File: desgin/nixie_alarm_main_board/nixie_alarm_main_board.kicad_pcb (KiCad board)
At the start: 2 copper layers, 138.2 x 53 mm, 105 parts, among them IC1 LM3488MM, IC2 HV5530PG-G, IC3 TPS563219ADDFR, IC4 HV5530PG-G, IC6 CD40109BQNSRQ1, IC7 AP7363-33D-13, IC8 MCP4018T-502E_LT, J1 PJ-094H-SMT-TR, J2 JST XH 2.54 3 pin, J3 USB_C_Receptacle_USB2.0_16P, Q1 SSM3K35AMFV,L3F, Q2 DMN60H080DS-13, Q3 DMN60H080DS-13, Q4 DMN60H080DS-13, Q5 DMN60H080DS-13, Q6 DMN60H080DS-13, Q7 DMN60H080DS-13, Q8 TPH5200FNH,L1Q, U1 ESP32-S3-WROOM-1

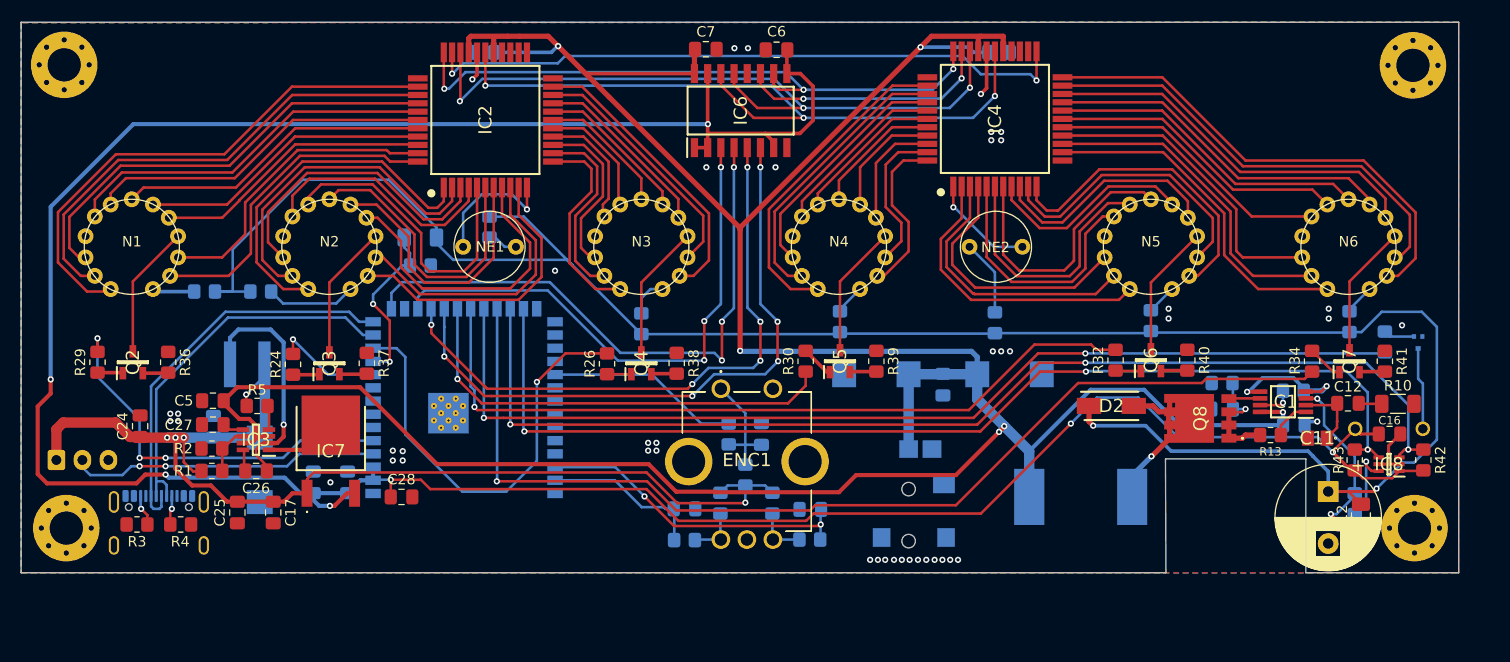
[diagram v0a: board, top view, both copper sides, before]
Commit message: add more detalis
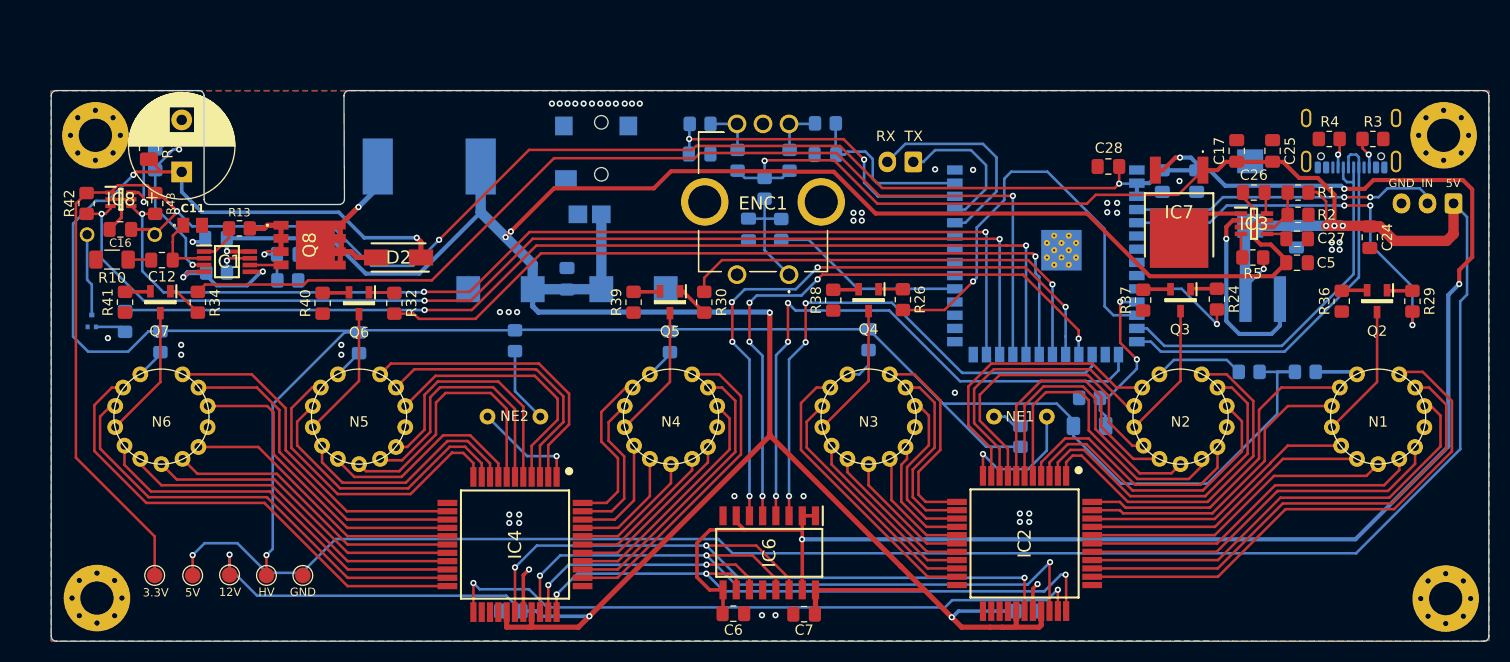
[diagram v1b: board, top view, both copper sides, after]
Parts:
- added 12V: TestPoint_Pad_D1.5mm, TestPoint:TestPoint_Pad_D1.5mm, F.Cu at (104.0, 120.2)
- added 3.3V: TestPoint_Pad_D1.5mm, TestPoint:TestPoint_Pad_D1.5mm, F.Cu at (96.8, 120.2)
- added 5V: TestPoint_Pad_D1.5mm, TestPoint:TestPoint_Pad_D1.5mm, F.Cu at (100.5, 120.2)
- added GND: TestPoint_Pad_D1.5mm, TestPoint:TestPoint_Pad_D1.5mm, F.Cu at (111.0, 120.2)
- added HV: TestPoint_Pad_D1.5mm, TestPoint:TestPoint_Pad_D1.5mm, F.Cu at (107.5, 120.2)
- added J4: JST XH 2.54 3 pin, Connector_JST:JST_EH_S2B-EH_1x02_P2.50mm_Horizontal, B.Cu at (169.8, 80.4)
- moved REF** 142.4 mm to (220.9, 122.4), turned to 180 degrees
- moved REF** 137.7 mm to (220.8, 77.9), turned to 180 degrees
- moved J2 136.6 mm to (221.7, 84.4), turned to 180 degrees
- moved REF** 136.5 mm to (91.2, 122.4), turned to 180 degrees
- moved REF** 132.4 mm to (91.1, 77.9), turned to 180 degrees
- moved R42 130.9 mm to (90.2, 84.4), turned to 90 degrees
- moved Q1 127.6 mm to (90.8, 95.7), turned to 180 degrees
- moved R29 126.6 mm to (217.8, 93.8), turned to -90 degrees
- moved IC8 124.6 mm to (93.5, 84.0), turned to 0 degrees
- moved R3 124.5 mm to (213.9, 78.2), turned to 0 degrees
- moved R10 124.4 mm to (92.7, 89.8), turned to 180 degrees
- moved C16 123.6 mm to (93.5, 86.9), turned to 180 degrees
- moved LS1 123.4 mm to (93.5, 87.4), turned to 180 degrees
- moved R12 122.1 mm to (96.2, 78.6), turned to 90 degrees
- moved R41 121.3 mm to (94.0, 93.9), turned to 90 degrees
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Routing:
- net +5V: track 111.0 -> 267.2 mm, vias 5 -> 6
- net +3.3V: track 282.8 -> 322.0 mm
- net +12V: track 288.7 -> 322.0 mm, vias 6 -> 7
- net HV: track 201.9 -> 229.7 mm, vias 2 -> 3
- net DEBUG_UART_RX: track 0.00 -> 20.3 mm
- net DEBUG_UART_TX: track 0.00 -> 14.2 mm
- net ENC_A: track 16.0 -> 17.3 mm
- net ENC_B: track 30.6 -> 31.8 mm
- net NX_DOT_6: track 101.7 -> 100.9 mm
- net GND: vias 47 -> 53
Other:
- outline, holes or cut-outs redrawn
- board text added: "5V"
- board text added: "GND"
- board text added: "HV Danger"
- board text added: "IN"
- board text added: "Nixie alarm clock"
- board text added: "Paderewski"
- board text added: "RX"
- board text added: "TX"
